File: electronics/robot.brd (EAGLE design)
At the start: 170.3 x 155.9 mm, 83 parts, among them J1 USB-B, J3 B6B-ZR, J4 B6B-ZR, J5 B6B-ZR, J6 KICKER, Q1 IRLMS2002TRPBF, Q2 IRLMS2002TRPBF, Q3 NPN_BC817,215, Q4 SUD50N04-8M8P-4GE3, Q5 NPN_BC817,215, Q6 NPN_BC817,215, U1 FT232L, U2 ESP32-WROOM-32E_(16MB), U3 S8252, U4 L9110, U5 L9110, U6 L9110, U7 MT3608

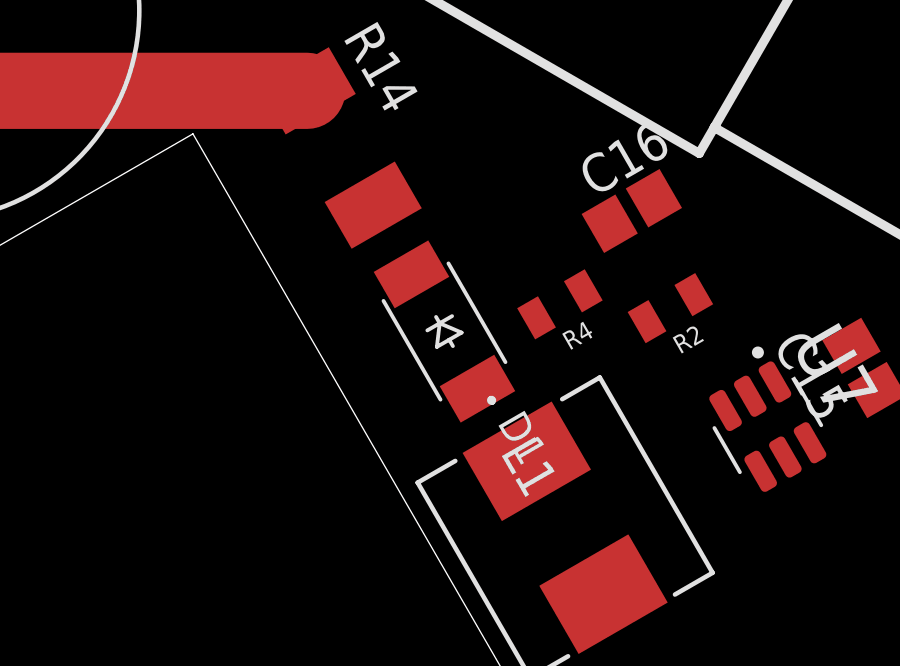
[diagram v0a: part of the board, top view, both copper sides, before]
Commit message: Minor fixes
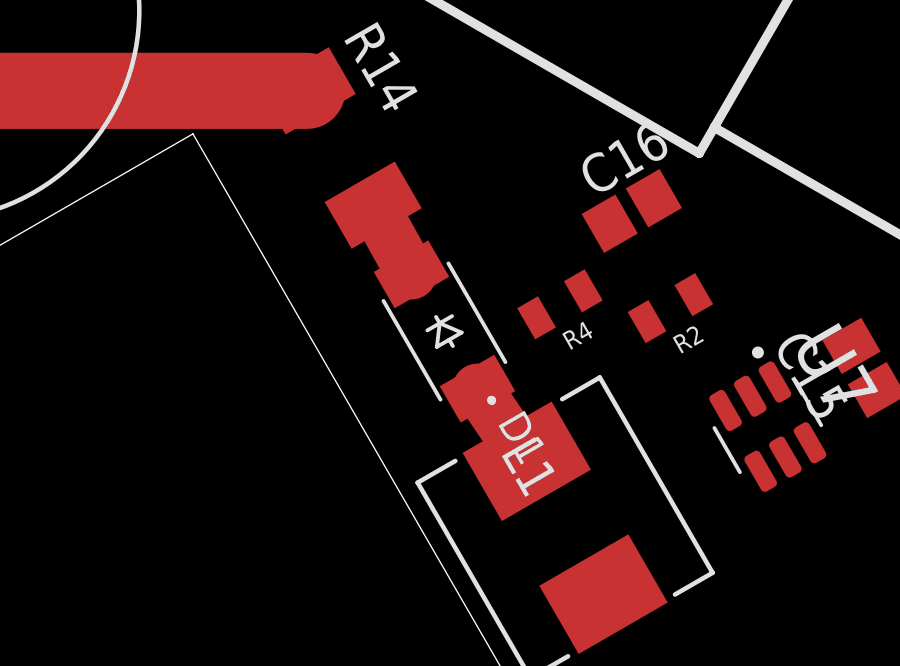
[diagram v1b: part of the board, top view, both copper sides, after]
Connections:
- removed net LEDS_SUITE: LED6.2-DOUT
- net GND: now also U1.26
- net M1C1: now also U2.26; no longer U2.23
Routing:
- net N$1: track 0.00 -> 2.93 mm
- net N$2: track 0.00 -> 2.64 mm
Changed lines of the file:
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@@
 <setting verticaltext="up"/>
 </settings>
-<grid distance="0.001" unitdist="inch" unit="inch" style="lines" multiple="2" display="yes" altdistance="0.25" altunitdist="mm" altunit="mm"/>
+<grid distance="0.0254" unitdist="mm" unit="mm" style="lines" multiple="2" display="yes" altdistance="0.25" altunitdist="mm" altunit="mm"/>
 <layers>
 <layer number="1" name="Top" color="4" fill="1" visible="yes" active="yes"/>
@@
 <contactref element="C13" pad="2"/>
 <contactref element="C14" pad="2"/>
+<contactref element="U1" pad="26"/>
 <wire x1="-66.09005625" y1="-32.6132375" x2="-68.94794375" y2="-34.2632375" width="0" layer="19" extent="1-16"/>
 <wire x1="-62.7435" y1="-33.1465875" x2="-66.09005625" y2="-32.6132375" width="0" layer="19" extent="1-1"/>
@@
 <wire x1="8.1444" y1="-40.82" x2="2.4794" y2="-35.155" width="0" layer="19" extent="1-1"/>
 <wire x1="12.885" y1="-36.505" x2="8.1444" y2="-40.82" width="0" layer="19" extent="1-1"/>
+<wire x1="20.135" y1="-33.905" x2="20.135" y2="-34.555" width="0" layer="19" extent="1-1"/>
 <wire x1="15.483" y1="-30.226" x2="17.3228" y2="-34.555" width="0" layer="19" extent="1-16"/>
 <wire x1="5.3594" y1="-23.31" x2="2.4794" y2="-31.485" width="0" layer="19" extent="1-1"/>
@@
 <wire x1="69.32894375" y1="-35.0252375" x2="-68.947940625" y2="-34.2632375" width="0" layer="19" extent="1-16"/>
 </signal>
-<signal name="LEDS_SUITE">
-<contactref element="LED6" pad="2-DOUT"/>
-</signal>
 <signal name="N$30">
 <contactref element="LED4" pad="2-DOUT"/>
@@
 <signal name="M1C1">
 <contactref element="J3" pad="4"/>
-<contactref element="U2" pad="23"/>
-<wire x1="-4.8006" y1="-23.31" x2="-18.7821125" y2="-31.239165625" width="0" layer="19" extent="1-1"/>
+<contactref element="U2" pad="26"/>
+<wire x1="-8.8556" y1="-25.58" x2="-18.7821125" y2="-31.239165625" width="0" layer="19" extent="1-1"/>
 </signal>
 <signal name="M1C2">
@@
 <contactref element="U7" pad="1"/>
 <contactref element="D1" pad="2"/>
-<wire x1="-45.05204375" y1="4.821184375" x2="-43.408521875" y2="2.40045625" width="0" layer="19" extent="1-1"/>
+<wire x1="-43.408521875" y1="2.40045625" x2="-45.05204375" y2="4.821184375" width="1.6764" layer="1"/>
 <wire x1="-35.136334375" y1="5.044246875" x2="-43.408521875" y2="2.40045625" width="0" layer="19" extent="1-1"/>
 </signal>
@@
 <contactref element="D1" pad="1"/>
 <contactref element="R14" pad="2"/>
-<wire x1="-48.527525" y1="10.938759375" x2="-47.252046875" y2="8.63169375" width="0" layer="19" extent="1-1"/>
+<wire x1="-47.252046875" y1="8.63169375" x2="-48.527525" y2="10.938759375" width="1.6764" layer="1"/>
 <wire x1="-43.082875" y1="7.18245" x2="-47.252046875" y2="8.63169375" width="0" layer="19" extent="1-1"/>
 <wire x1="-40.6435875" y1="10.318953125" x2="-43.082875" y2="7.18245" width="0" layer="19" extent="1-1"/>
